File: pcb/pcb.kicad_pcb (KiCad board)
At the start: 2 copper layers, 100 x 88.7 mm, 65 parts, among them J1 AudioJack4, J2 USB_C_Receptacle_USB2.0, SW1 Switch, SW10 Switch, SW11 Switch, SW12 Switch, SW13 Switch, SW14 Switch, SW15 Switch, SW16 Switch, SW17 Switch, SW18 Switch, SW2 Switch, SW3 Switch, SW4 Switch, SW5 Switch, SW6 Switch, SW7 Switch, SW8 Switch, SW9 Switch, U1 MCU_rp2040-zero, U2 MCU_rp2040-zero, U3 RollerEncoder_EVQWGD001

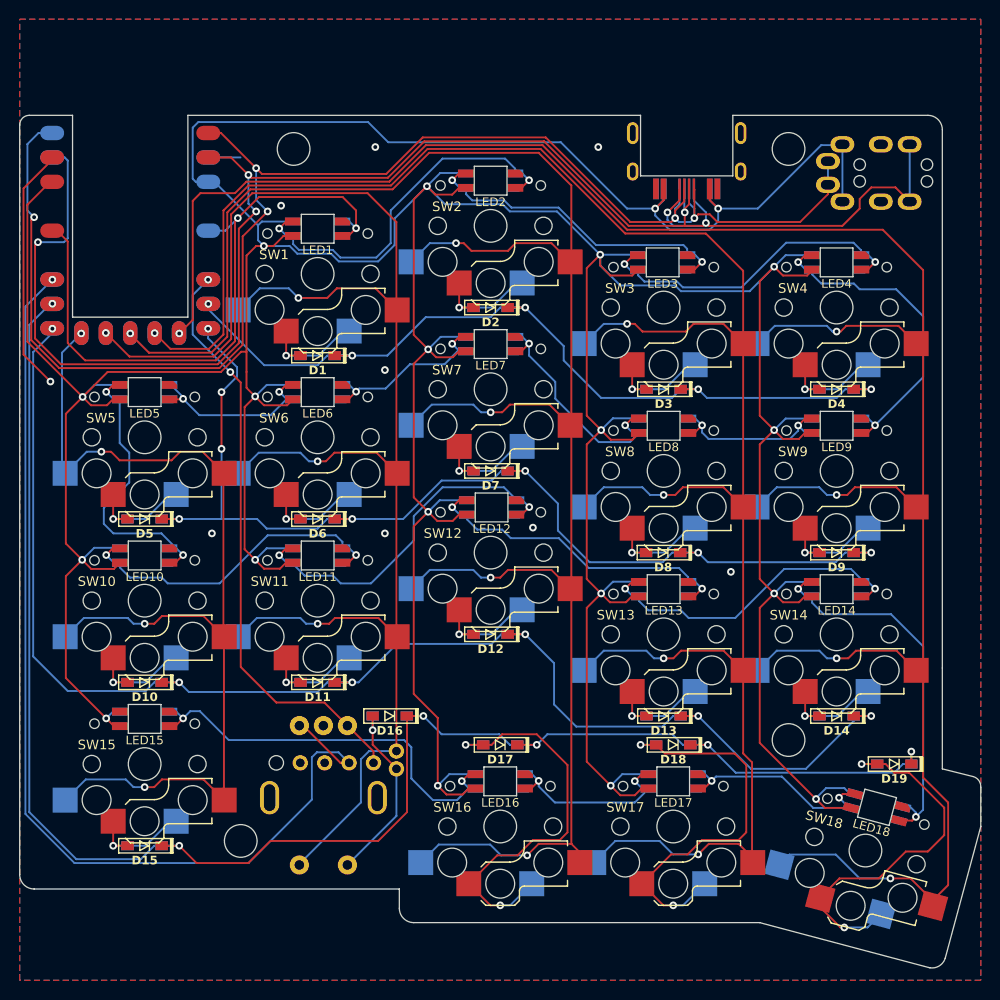
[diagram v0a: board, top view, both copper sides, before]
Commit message: new pcb
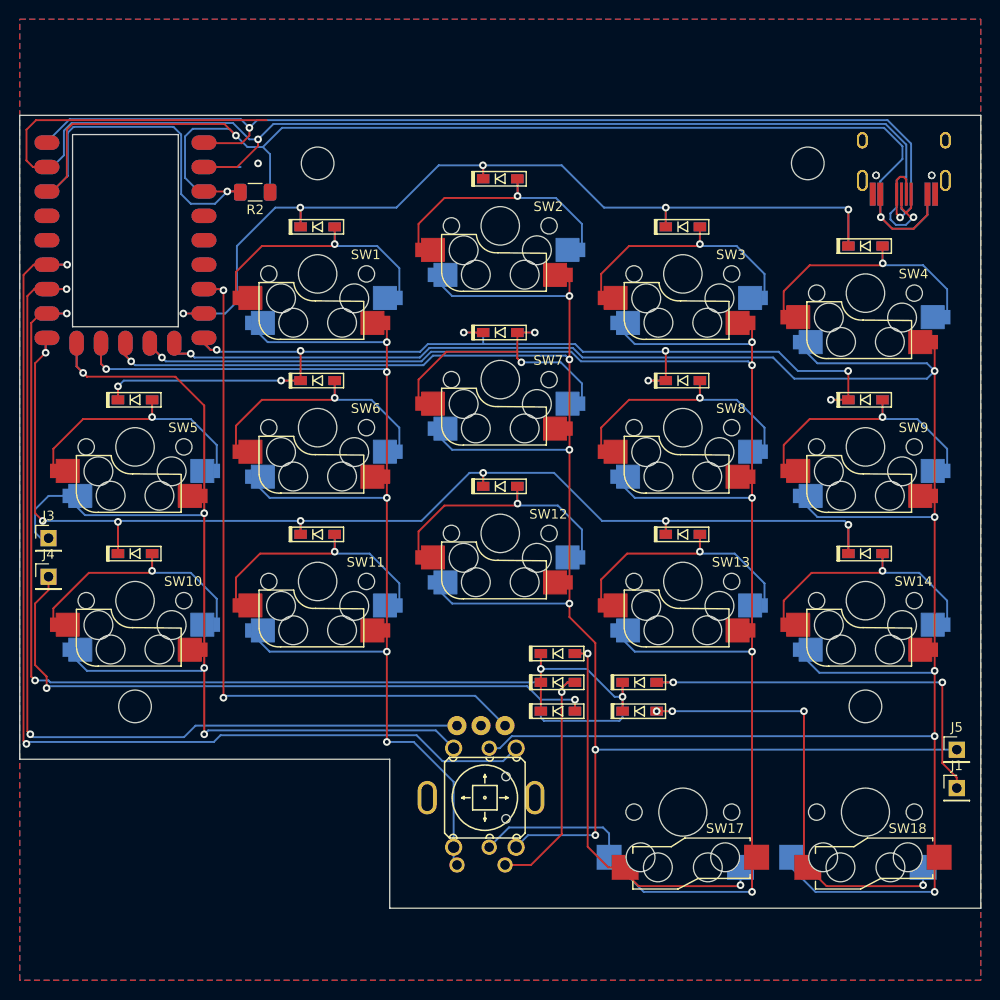
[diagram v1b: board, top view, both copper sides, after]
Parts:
- removed J2: USB_C_Receptacle_USB2.0, zzkeeb:Connector_USB-C-mid-mount-ali-reversible-data
- removed LED1, LED10, LED11, LED12, LED13, LED14, LED15, LED16, LED17, LED18, LED2, LED3, LED4, LED5, LED6, LED7, LED8, LED9: LED_SK6812MINI-E, zzkeeb:LED_SK6812-MINI-E-reversible
- removed SW15, SW16: Switch, zzkeeb:Switch_ChocV1-hotswap-reversible
- removed U3: RollerEncoder_EVQWGD001, zzkeeb:RotaryEncoder_EVQWGD001
- added FiveWay1: 5Way-Tactile_K1-1506DN-01, zzkeeb:Button_5way, F.Cu at (100.9, 111.5)
- added J3: C0, Connector_PinHeader_2.54mm:PinHeader_1x01_P2.54mm_Vertical, F.Cu at (55.5, 84.5)
- added J4: R3, Connector_PinHeader_2.54mm:PinHeader_1x01_P2.54mm_Vertical, F.Cu at (55.5, 88.5)
- added J5: C2, Connector_PinHeader_2.54mm:PinHeader_1x01_P2.54mm_Vertical, F.Cu at (150.0, 106.5)
- added R1: 4.7k, Resistor_SMD:R_1206_3216Metric_Pad1.30x1.75mm_HandSolder, B.Cu at (77.0, 48.5)
- added R2: 4.7k, Resistor_SMD:R_1206_3216Metric_Pad1.30x1.75mm_HandSolder, F.Cu at (77.0, 48.5)
- added USB1: Connector_HRO-TYPE-C-31-M-12, zzkeeb:Connector_HRO-TYPE-C-31-M-12-data, B.Cu at (144.5, 40.5)
- added USB2: Connector_HRO-TYPE-C-31-M-12, zzkeeb:Connector_HRO-TYPE-C-31-M-12-data, F.Cu at (144.5, 40.5)
- D1, D10, D11, D12, D13, D14, D15, D16, D17, D18, D19, D2, D3, D4, D5, D6, D7, D8, D9: footprint zzkeeb:Diode_1N4148-SOD123-reversible-flip3d -> zzkeeb:Diode_1N4148-SOD123-no-label-reversible-flip3d
- J1: value AudioJack4 -> R3; footprint zzkeeb:Connector_TRRS-reversible -> Connector_PinHeader_2.54mm:PinHeader_1x01_P2.54mm_Vertical
- SW1, SW10, SW11, SW12, SW13, SW14, SW2, SW3, SW4, SW5, SW6, SW7, SW8, SW9: footprint zzkeeb:Switch_ChocV1-hotswap-reversible -> zzkeeb:Switch_MX-hotswap-miny-reversible
- SW17, SW18: footprint zzkeeb:Switch_ChocV1-hotswap-reversible -> zzkeeb:Switch_KS-miny-reversible-hotswap-south
- moved J1 64.0 mm to (150.0, 110.5), turned to 0 degrees
- moved D15 54.2 mm to (117.0, 99.5), turned to 0 degrees
- moved D19 27.1 mm to (117.0, 102.5), turned to 0 degrees
- moved D13 19.0 mm to (121.5, 84.1), turned to 0 degrees
- moved D8 18.0 mm to (121.5, 68.1), turned to 0 degrees
- moved D16 17.8 mm to (108.5, 99.5), turned to 0 degrees
- moved H3 17.8 mm to (64.5, 102.0)
- moved D14 17.2 mm to (140.5, 86.1), turned to 0 degrees
- moved D3 17.0 mm to (121.5, 52.1), turned to 0 degrees
- moved RE1 16.4 mm to (100.5, 111.5)
- moved D9 16.2 mm to (140.5, 70.1), turned to 0 degrees
- moved D12 15.4 mm to (102.5, 79.1), turned to 0 degrees
- moved D11 15.4 mm to (83.5, 84.1), turned to 0 degrees
- moved D18 15.3 mm to (108.5, 96.5), turned to 0 degrees
- moved D4 15.2 mm to (140.5, 54.1), turned to 0 degrees
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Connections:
- D15 pad 2: Net-(D15-Pad2) -> Net-(D15-A)
- U1 pad 19: LED -> unconnected-(U1-28-Pad19)
- U2 pad 19: LED -> unconnected-(U2-28-Pad19)
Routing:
- net VCC: track 635.8 -> 138.4 mm, vias 20 -> 2
- net row4: track 0.00 -> 108.5 mm, vias 0 -> 2
- net LED: track 67.4 -> 0.00 mm, vias 2 -> 0
- net RX: track 171.9 -> 120.3 mm, vias 6 -> 2
- net row3: track 175.1 -> 130.5 mm, vias 6 -> 4
- net Net-(LED15-Pad4): track 44.0 -> 0.00 mm, vias 2 -> 0
- net TX: track 159.1 -> 116.1 mm, vias 5 -> 2
- net Net-(D15-A): track 0.00 -> 43.1 mm, vias 0 -> 2
- net Net-(LED14-Pad2): track 39.7 -> 0.00 mm, vias 2 -> 0
- net Net-(LED1-Pad2): track 38.8 -> 0.00 mm, vias 2 -> 0
- net Net-(LED11-Pad2): track 37.3 -> 0.00 mm, vias 2 -> 0
- net hand: track 0.00 -> 36.9 mm, vias 0 -> 1
- net Net-(LED4-Pad2): track 34.5 -> 0.00 mm, vias 2 -> 0
- net col1: track 177.5 -> 143.2 mm, vias 4 -> 6
- net Net-(LED10-Pad2): track 34.4 -> 0.00 mm, vias 2 -> 0
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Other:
- board size 100 x 88.7 mm -> 100 x 82.5 mm
